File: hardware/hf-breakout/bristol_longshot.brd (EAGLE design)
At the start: 31 x 50 mm, 22 parts, among them U1 SAM_D20E

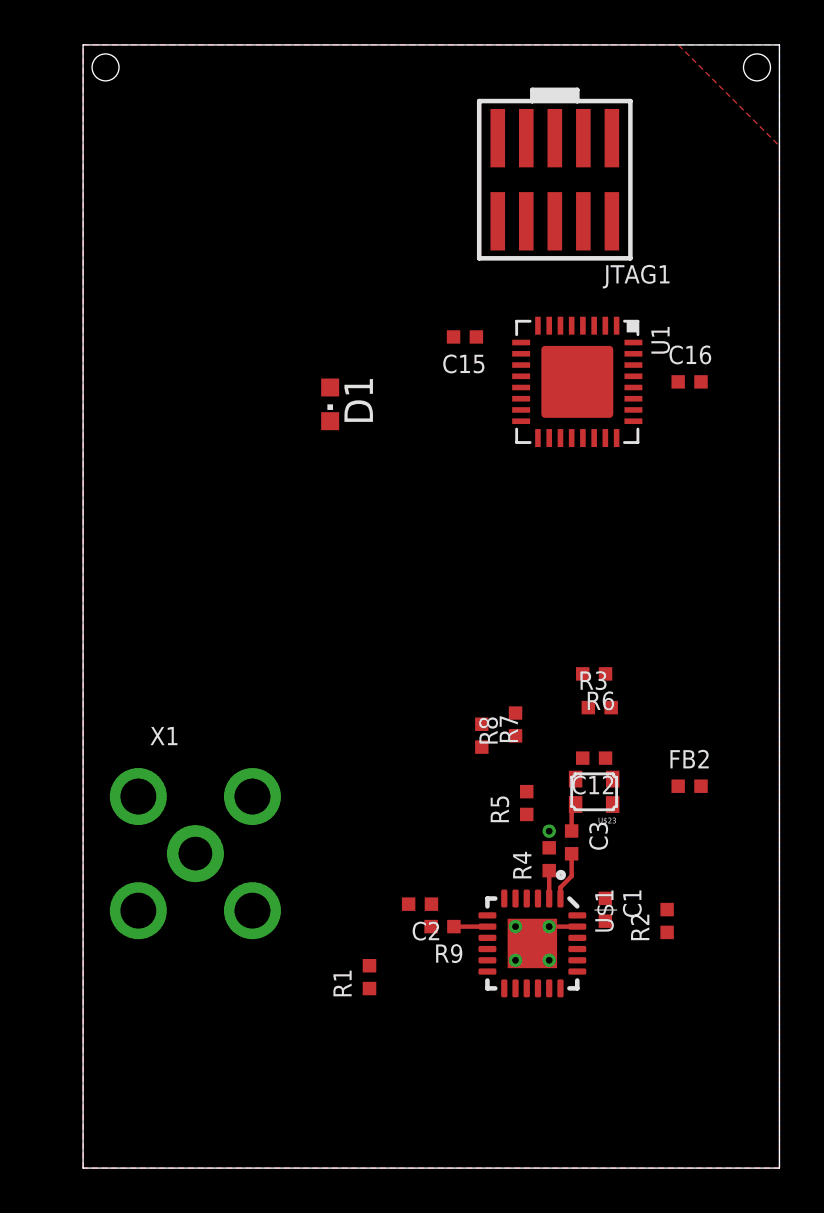
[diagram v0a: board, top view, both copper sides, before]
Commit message: HF board done
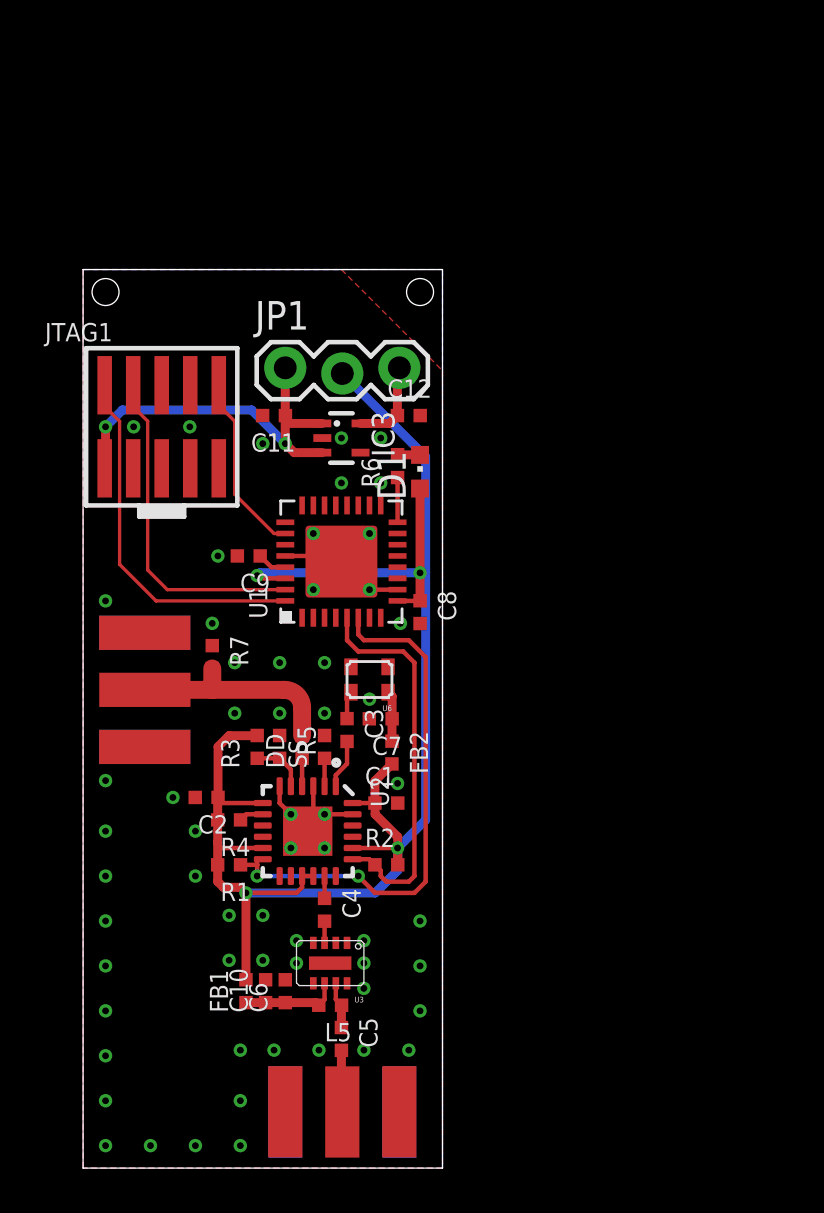
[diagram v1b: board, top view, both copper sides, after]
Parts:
- removed C15, C16: 100nF, microbuilder_v3:_0402
- removed R8, R9: 10kΩ, microbuilder_v3:_0402
- removed U$1: SI5356, si5356:QFN24_4MM
- removed U$23: TG-5006CJ, fbri:TC-5006CJ
- removed X1: (no value), microbuilder_v3:SMA90_DIP
- added C10: 100pF, microbuilder_v3:_0402
- added C11: 1µF, microbuilder_v3:_0402
- added C4, C5, C6, C7, C8, C9: 100nF, microbuilder_v3:_0402
- added DD, SS: 0Ω, microbuilder_v3:_0402
- added FB1: (no value), microbuilder_v3:_0402
- added IC3: TLV70018DCK, tlv700:SC70-5L
- added J$1, J$2: SMA_EDGE, SparkFun:SMA-EDGE
- added JP1: (no value), SparkFun:1X03_LOCK
- added L5: 100nH, microbuilder_v3:_0402
- added U2: SI5356, si5356:QFN24_4MM
- added U3: AD8354, fbri:LFCSP_VD_8
- added U6: TG-5006CJ, fbri:TC-5006CJ
- C12: value 100nF -> 1µF
- R4: value 0Ω -> 10kΩ
- R5: value 0Ω -> 15kΩ
- R6: value 15kΩ -> 220Ω
- R7: value 15kΩ -> DNP
- moved JTAG1 20.7 mm to (3.50, 33.0), turned to 0 degrees
- moved C12 17.3 mm to (14.5, 33.5), turned to 0 degrees
- moved R3 15.4 mm to (7.75, 18.8), turned to 90 degrees
- moved R4 14.4 mm to (6.50, 15.5), turned to 180 degrees
- moved FB2 13.3 mm to (13.8, 18.5), turned to 270 degrees
- moved U1 13.2 mm to (11.5, 27.0), turned to 90 degrees
- moved R2 12.7 mm to (13.5, 13.5), turned to 0 degrees
- moved R6 12.7 mm to (14.0, 31.2), turned to 90 degrees
- moved R7 12.5 mm to (5.75, 22.8)
- moved R5 11.3 mm to (8.75, 18.8), turned to 270 degrees
- moved C3 11.2 mm to (11.8, 19.5)
- moved C1 10.8 mm to (13.5, 16.2), turned to 0 degrees
- moved C2 10.6 mm to (5.50, 16.5)
- moved R1 8.00 mm to (6.50, 13.5), turned to 180 degrees
- moved D1 5.00 mm to (15.0, 31.0), turned to 0 degrees
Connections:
- removed net !OE: R7.2, R8.1, U$1.6
- removed net !OE_CTRL: R8.2
- new net 3.3V: C11.1, IC3.1, IC3.3, JP1.1, JTAG1.1
- new net AMPL_OUT: C5.1, L5.1, U3.7
- new net AMPL_VPOS: C10.1, C6.1, FB1.1, L5.2, U3.6
- new net HF: C5.2, J$2.SIG
- new net HF_CLK: C4.1, U2.17
- new net INPT: C4.2, U3.3
- new net LED_R: R6.1, U1.16
- new net N$1: C12.1, IC3.5, JP1.3
- net 1.8V: now also C8.1, FB1.2, JP1.2, R4.2, U2.11, U2.15, U2.16, U2.20, U2.24, U2.7; no longer C15.1, JTAG1.1, R9.2, U$1.11, U$1.15, U$1.16, U$1.20, U$1.24, U$1.7
- net CLKIN: now also DD.1, U2.4; no longer R5.1, U$1.4
- net CLKIN_SMA: now also DD.2, J$1.SIG, R7.2; no longer R5.2, X1.ANTENNA
- net GND: now also C10.2, C11.2, C6.2, C7.2, C8.2, C9.2, IC3.2, J$1.GND@0, J$1.GND@1, J$1.GND@2, J$1.GND@3, J$2.GND@0, J$2.GND@1, J$2.GND@2, J$2.GND@3, R5.1, SS.2, U2.23, U2.3, U2.6, U2.PAD, U3.1, U3.4, U3.5, U3.8, U3.EPAD, U6.2; no longer C15.2, C16.2, R4.2, R6.1, U$1.23, U$1.3, U$1.PAD, U$23.2, X1.GND1, X1.GND2, X1.GND3, X1.GND4
- net INTR: now also R4.1, U2.8; no longer R9.1, U$1.8
- net LED: now also R6.2; no longer U1.16
- net SCL: now also U1.6, U2.12; no longer U$1.12
- net SDA: now also U1.5, U2.19; no longer U$1.19
- net SSC_DIS: now also R5.2, U2.5; no longer R6.2, U$1.5
- net TCXO_OUT: now also U6.3; no longer U$23.3
- net TCXO_VDD: now also C7.1, U6.4; no longer C12.1, U$23.4
- net VDD_CORE: now also C9.1; no longer C16.1
- net XA: now also U2.1; no longer U$1.1
- net XB: now also SS.1, U2.2; no longer R4.1, U$1.2
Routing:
- net 1.8V: track 0.00 -> 75.8 mm, vias 0 -> 4
- net SCL: track 0.00 -> 23.9 mm, vias 0 -> 2
- net 3.3V: track 0.00 -> 18.0 mm, vias 0 -> 2
- net SDA: track 0.00 -> 17.3 mm
- net SWDIO: track 0.00 -> 16.3 mm
- net SWDCLK: track 0.00 -> 15.0 mm
- net CLKIN_SMA: track 0.00 -> 9.52 mm
- net GND: track 1.25 -> 10.4 mm, vias 5 -> 60
- net !RESET: track 0.00 -> 8.12 mm
- net AMPL_VPOS: track 0.00 -> 4.37 mm
- net N$1: track 0.00 -> 3.95 mm
- net HF: track 0.00 -> 2.76 mm
- net SSC_DIS: track 0.00 -> 2.45 mm
- net TCXO_VDD: track 0.00 -> 2.26 mm
- net AMPL_OUT: track 0.00 -> 2.08 mm
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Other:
- board size 31 x 50 mm -> 16 x 40 mm
- board text added: "1.8V"
- board text added: "3.3V"
- board text added: "ARM-SWD"
- board text added: "CLKIN"
- board text added: "HF OUT"
